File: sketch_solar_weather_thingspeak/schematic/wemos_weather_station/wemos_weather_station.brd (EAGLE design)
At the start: 45.7 x 61.9 mm, 10 parts, among them U1 PHOTORESISTOR-5528-10K

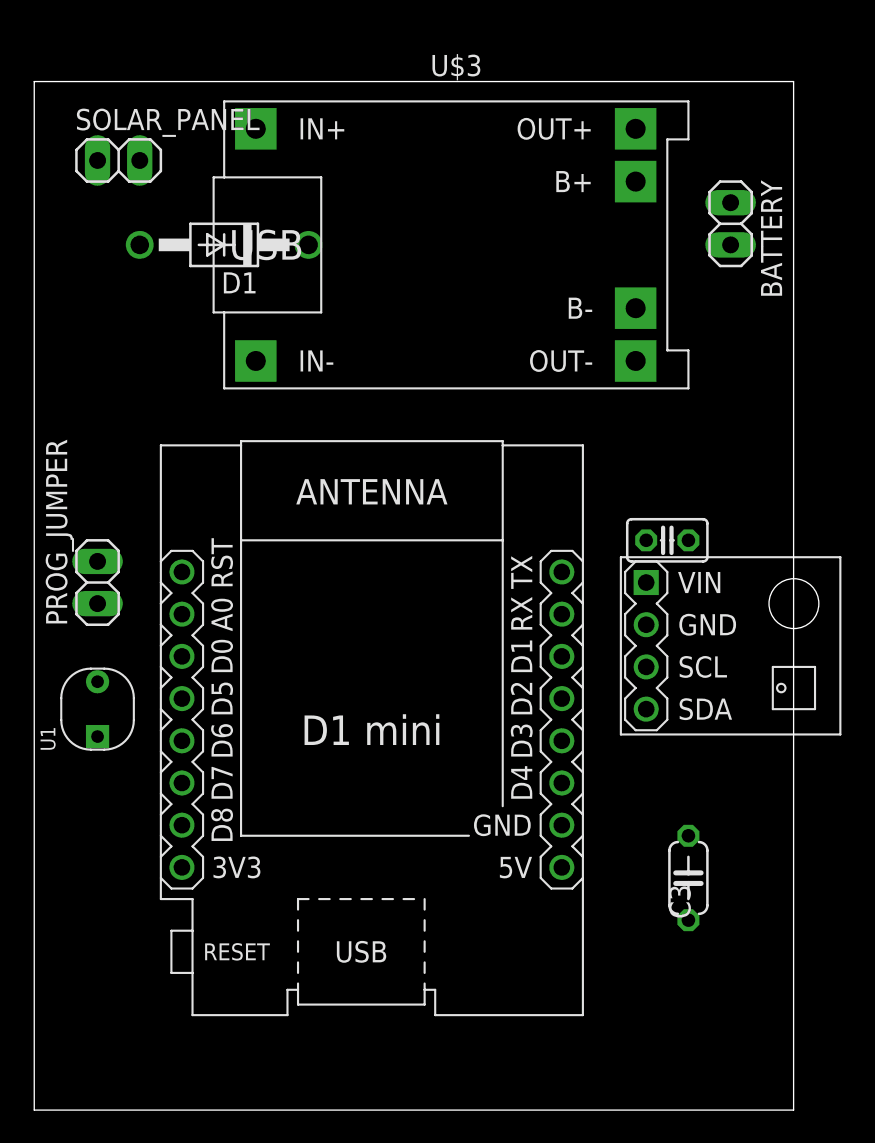
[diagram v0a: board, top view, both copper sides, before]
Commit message: Schematic updated
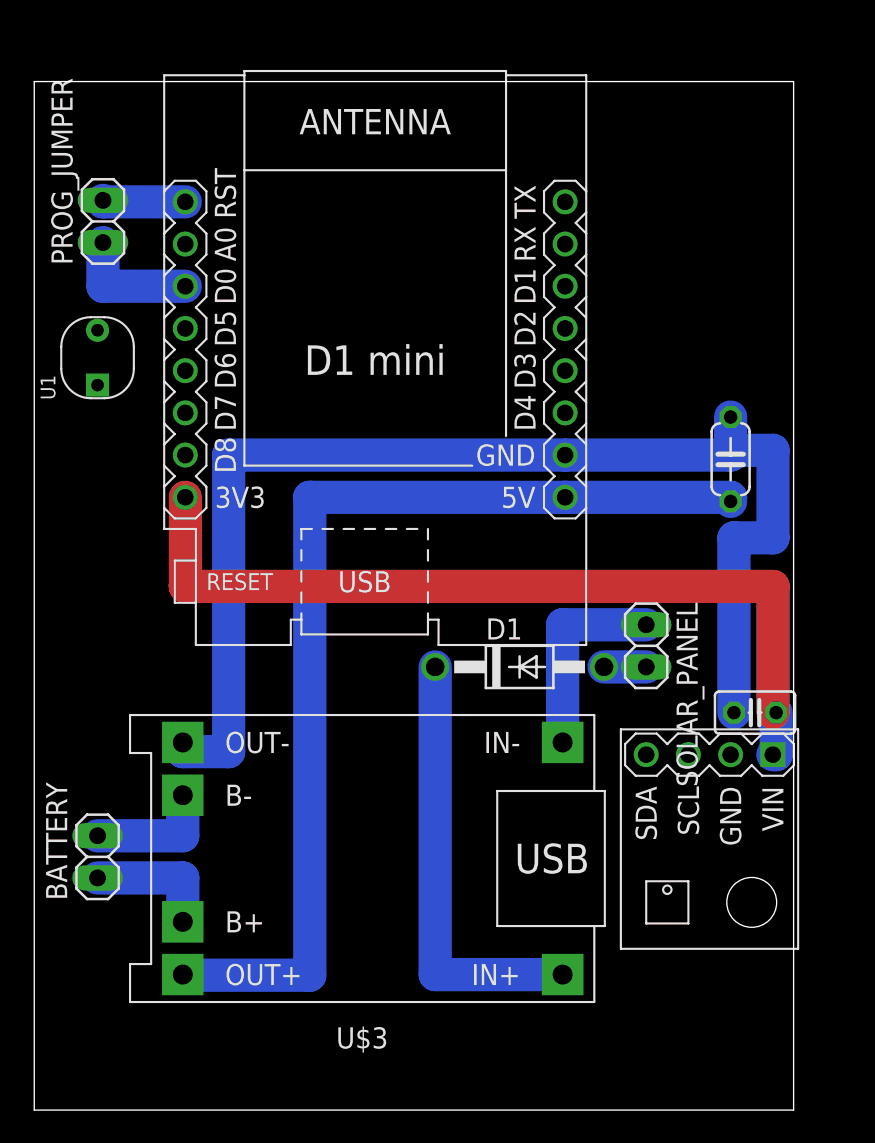
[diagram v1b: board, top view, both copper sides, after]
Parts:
- moved BATTERY 53.9 mm to (3.81, 53.3), turned to 90 degrees
- moved SOLAR_PANEL 43.1 mm to (36.8, 66.0), turned to 270 degrees
- moved U$3 37.4 mm to (19.7, 53.2), turned to 180 degrees
- moved D1 31.0 mm to (29.2, 64.8), turned to 0 degrees
- moved C3 25.3 mm to (41.9, 77.3)
- moved U$2 22.3 mm to (20.5, 83.2)
- moved PROG_JUMPER 21.7 mm to (4.13, 91.6)
- moved U1 21.1 mm to (3.81, 83.4)
- moved U$1 11.7 mm to (40.6, 54.4), turned to 270 degrees
- moved C1 11.6 mm to (43.4, 62.0)
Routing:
- net GNDA: track 0.00 -> 73.6 mm
- net VCC: track 0.00 -> 62.0 mm
- net N$7: track 0.00 -> 51.1 mm
- net N$2: track 0.00 -> 26.2 mm
- net N$1: track 0.00 -> 12.1 mm
- net N$3: track 0.00 -> 7.77 mm
- net N$6: track 0.00 -> 7.58 mm
- net N$4: track 0.00 -> 7.57 mm
- net N$10: track 0.00 -> 5.04 mm
- net N$5: track 0.00 -> 2.54 mm
